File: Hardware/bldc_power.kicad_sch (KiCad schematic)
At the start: 48 parts, among them U2 TC2117, U3 DRV8302

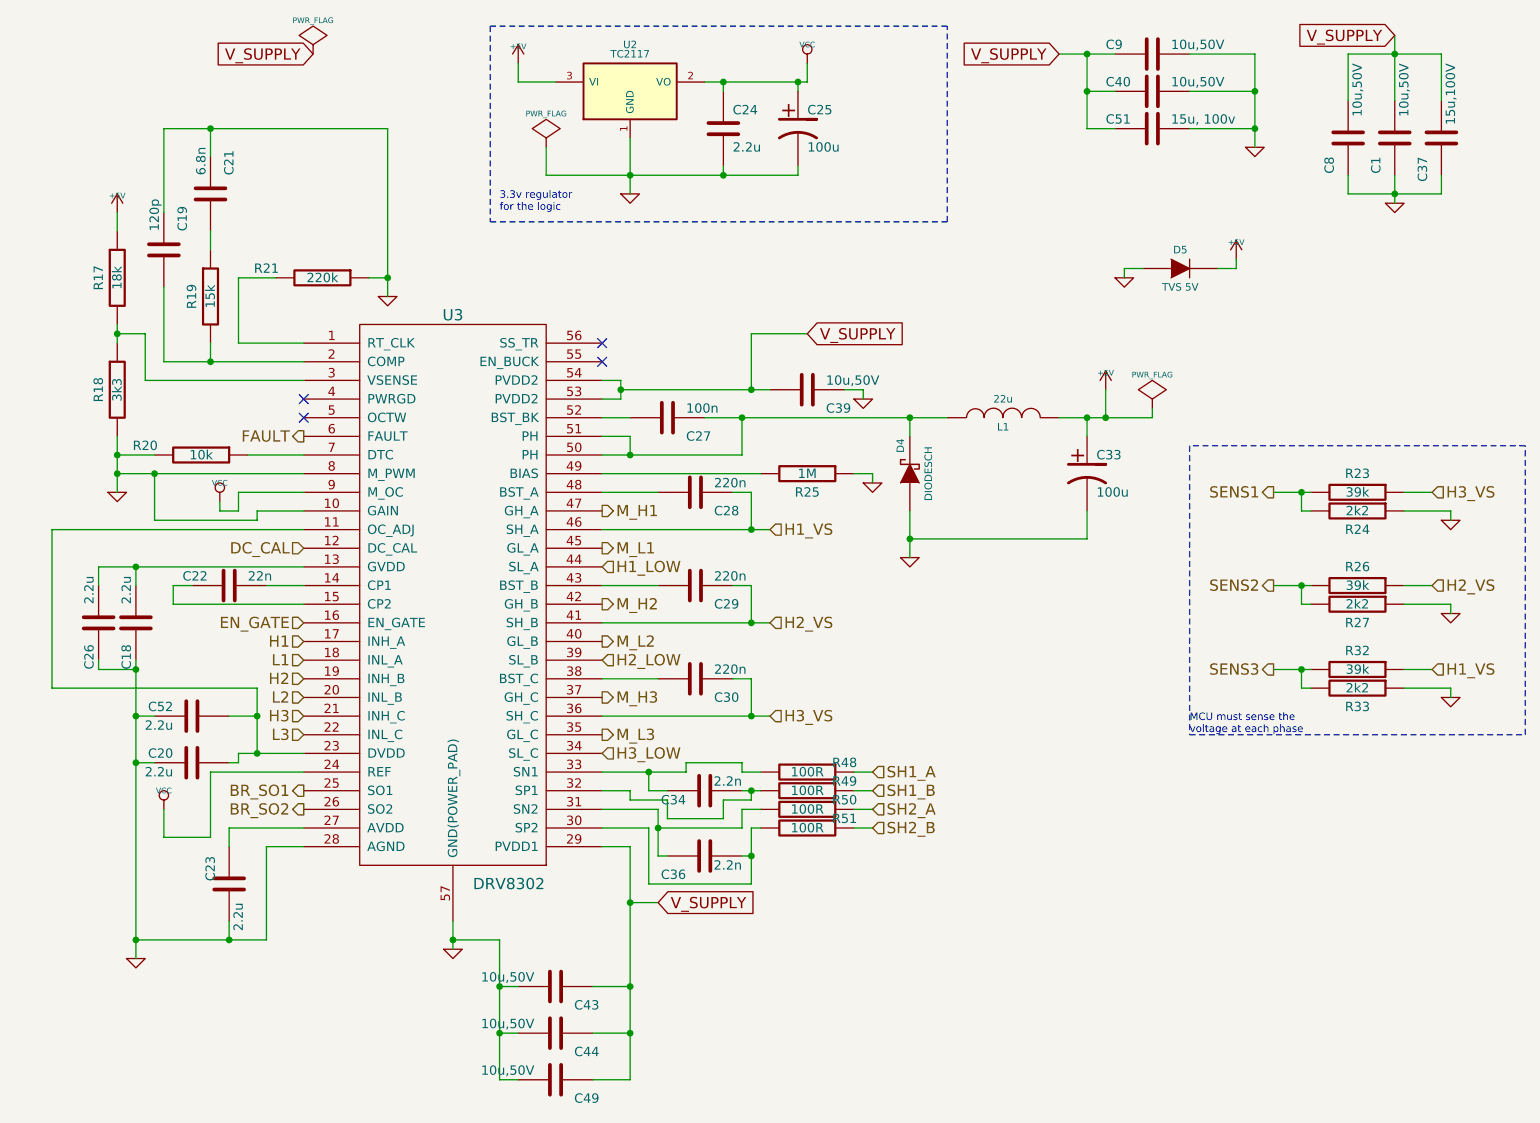
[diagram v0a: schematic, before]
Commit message: chatting to fang
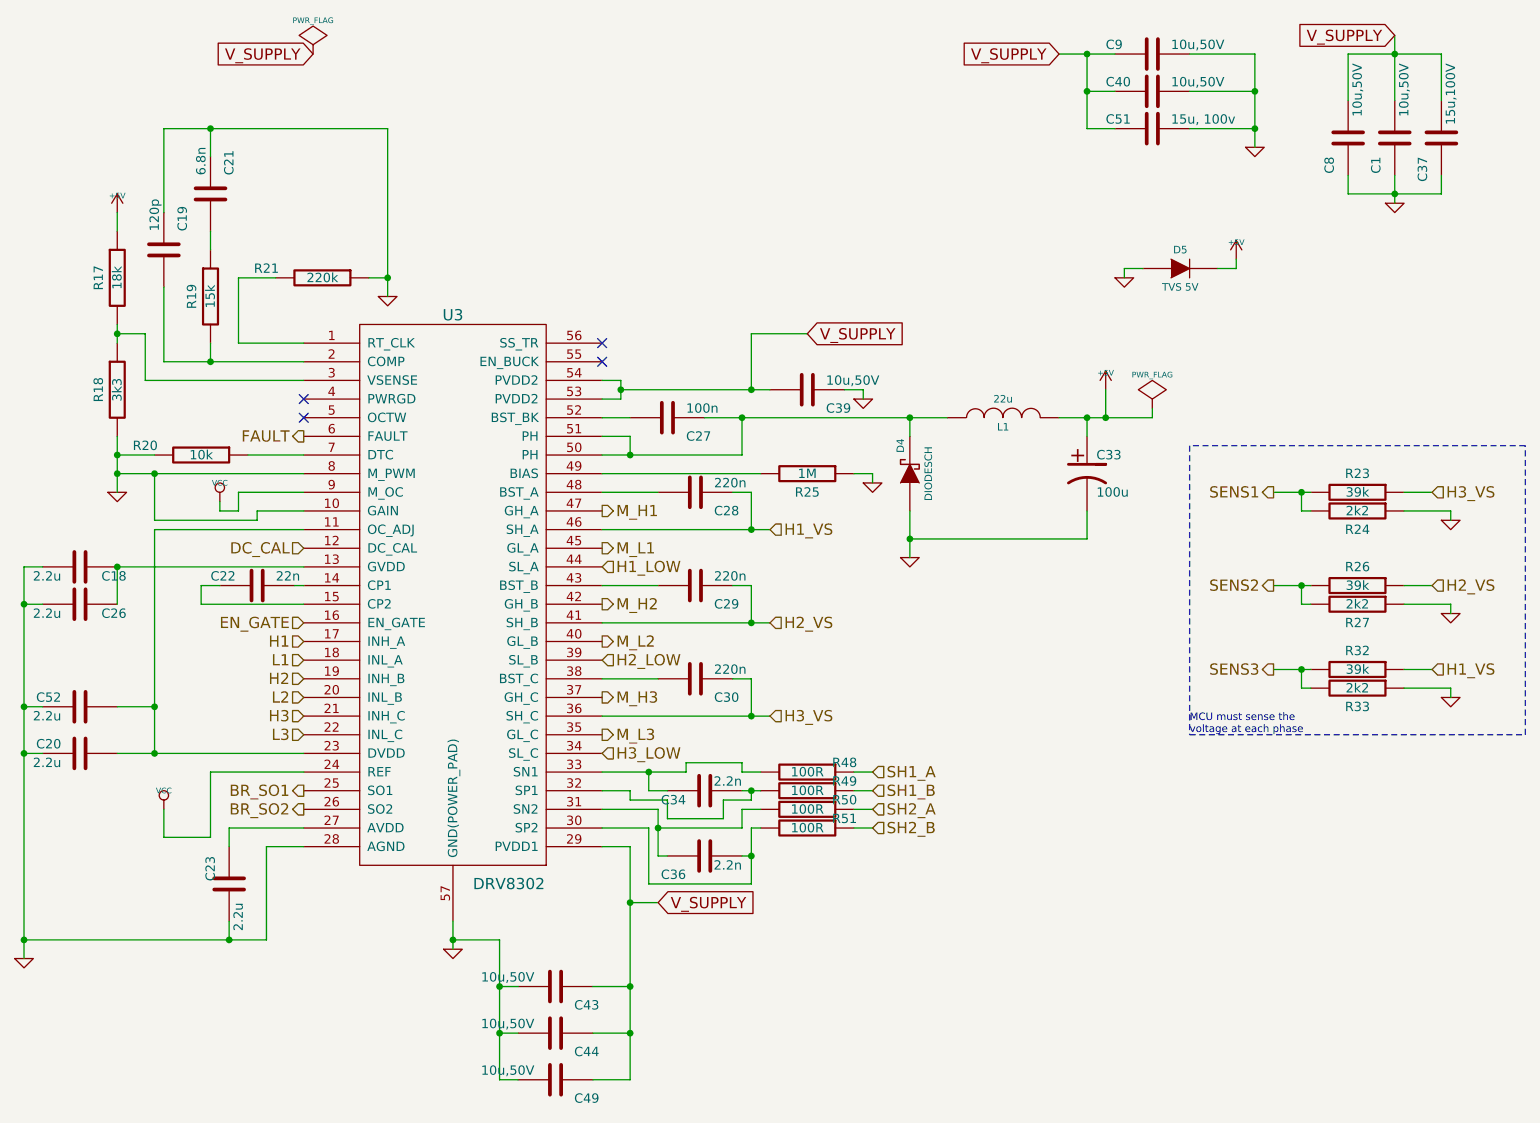
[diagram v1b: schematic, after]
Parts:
- removed C24: 2.2u, CRF1:SMD-0603_c, symbol BLDC_4-rescue:C-RESCUE-BLDC_4
- removed C25: 100u, w_smd_cap:c_tant_B, symbol BLDC_4-rescue:CP1-RESCUE-BLDC_4
- removed U2: TC2117, CRF1:SOT-223, symbol BLDC_4-rescue:NCP1117ST33T3G
- C1, C39, C40, C43, C44, C49, C8, C9: footprint CRF1:SMD-1206 -> Capacitor_SMD:C_1206_3216Metric
- C18, C19, C20, C21, C22, C23, C26, C27, C28, C29, C30, C34, C36, C52: footprint CRF1:SMD-0603_c -> Capacitor_SMD:C_0603_1608Metric
- C37, C51: footprint w_smd_cap:c_2220 -> Capacitor_SMD:C_2220_5750Metric
- R17, R18, R19, R20, R21, R24, R27, R33: footprint CRF1:SMD-0603_r -> Resistor_SMD:R_0402_1005Metric
- R23, R25, R26, R32, R48, R49, R50, R51: footprint CRF1:SMD-0603_r -> Resistor_SMD:R_0603_1608Metric
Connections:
- net GND: now also C18.1, C26.1; no longer C18.2, C26.2
- new net: C18.2, C26.2, U3.13 (GVDD)
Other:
- note removed: "3.3v regulator for the logic"
- moved on the sheet: C18, C20, C22, C26, C52
